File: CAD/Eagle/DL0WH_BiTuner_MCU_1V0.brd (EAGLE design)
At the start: 96.5 x 96.5 mm, 526 parts, among them Q0321 ABS07-32.768KHZ, Q1321 ABS07-32.768KHZ, Q2211 ABM3B-32.0000MHZ, Q2311 ABM3B-16.0000MHZ, T1051 MMBT2222, T1111 MMBT2222, T1121 MMBT2222, T1131 MMBT2222, U0111 STM32L4Z_144PIN_SMPS, U0521 PCAL6416APW, U0621 PCAL6416APW, U0711 IS25LP032D, U0721 IS25LP032D, U0801 CAT24C64, U0911 ZIO_EINK_1IN54, U1001 MIDAS_MCCOG21605B6W-FPTLWI, U1301 BNO085, U1401 BME680, U1501 LM4120IM5-3.0, U1511 MAX5217, U1531 CFPT-141-20MHZ, U1541 OPA354, U1542 LPV811, U1601 Si5338, U1651 TS5A23166, U1701 PCM1863, U1801 WM8523, U1901 SIM868, U2001 74LVC4245A, U2101 74LVC4245A, U2201 SX1262, U2271 PE4259, U2301 AX5243, U2401 LM53603-Q1, U2501 BQ24193, U2541 LPV811, U2601 BQ25570, U2681 TS5A23166, U2701 TPS62051, U2751 MCP4661-104E-MS, U2801 TS5A23166, U2901 TS5A23166, U3001 TS5A23166, U3101 TS5A23166, U3391 TS5A23166, U3392 TDK B4310, X1201 TTE_EN11-HSM, X1951 MICROSIM-8P_SDCARD-8P_MOLEX-1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, X2411 WIRE-TO-BOARD_5MM08_1X02, X2551 JST_S3B-XH-A, X2601 WIRE-TO-BOARD_5MM08_1X02, X3201 MOLEX 105017-0001, X3301 SMA_SMT_AMPHENOL-901-143, X3311 SAMTEC SMA-J-P-H-RA-TH1, X3371 SMA_SMT_AMPHENOL-901-143, SAM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, X3381 SMA_SMT_AMPHENOL-901-143, SAM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, X3391 SMA_SMT_AMPHENOL-901-143, SAM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, X3401 CUI SJ1-3535NS, X3411 CUI SJ1-3535NS, X3511 2X20/90_1MM27_HARWIN_M50-3202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, X3512 2X20/90_1MM27_HARWIN_M50-3202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, X3531 2X20/90_1MM27_HARWIN_M50-3202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, X3532 2X20/90_1MM27_HARWIN_M50-3202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

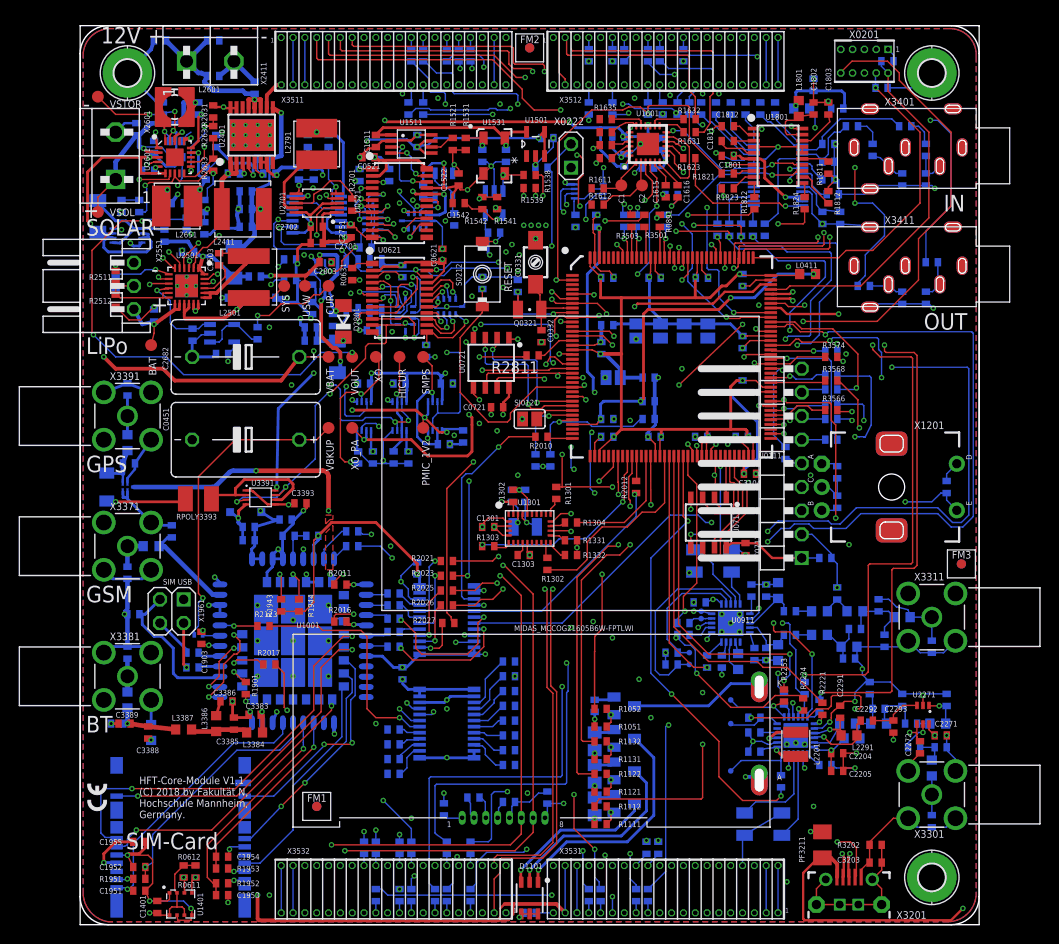
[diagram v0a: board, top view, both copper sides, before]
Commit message: HW_1V0 - CAD/Eagle - Initial setup of new PCB
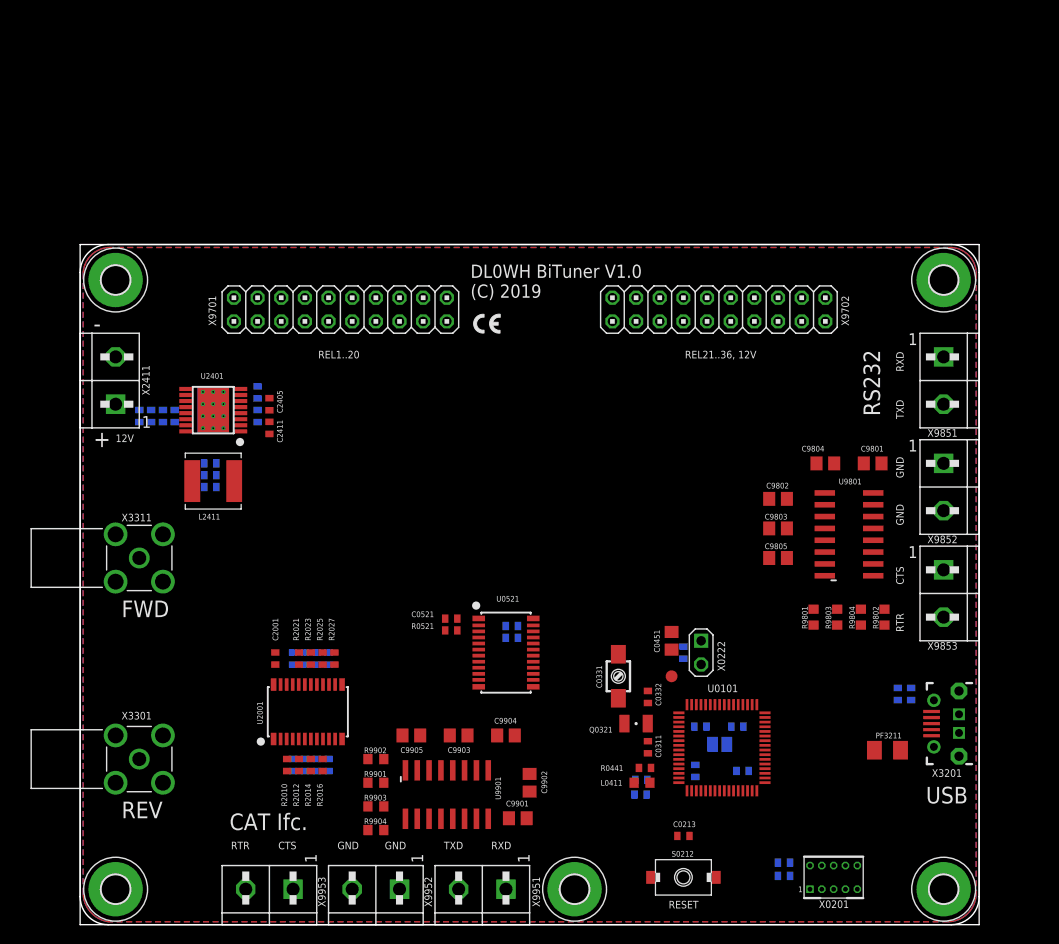
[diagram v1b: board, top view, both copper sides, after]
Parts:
- removed C0404, C0405, C0406, C0407, C0408, C0409, C0421, C0422, C0441, C0621, C0901, C1001, C1101, C1301, C1302, C1303, C1401, C1501, C1511, C1512, C1531, C1541, C1543, C1602, C1603, C1605, C1702, C1703, C1705, C1902, C2101, C2202, C2271, C2301, C2302, C2303, C2541, C2602, C2702, C2751, C2801, C2802, C2803, C2901, C2902, C2903, C3001, C3002, C3003, C3101, C3102, C3103, C3104, C3105, C3393: 100nF, df4iah_rcl:C0402
- removed C0423, C1801, C1802, C2606: 4.7uF, df4iah_rcl:C0402
- removed C0442, C1011, C1012, C1522, C1811, C1812, C1961, C2502, C2521: 1uF, df4iah_rcl:C0402
- removed C0711, C0721, C0801, C1601, C1604, C1951, C1955: 220nF, df4iah_rcl:C0402
- removed C1201, C1202, C1203, C1542, C2272: 1nF, df4iah_rcl:C0402
- removed C1321, C1322, C1952, C1953, C1954: 22pF, df4iah_rcl:C0402
- removed C1532: 100pF, df4iah_rcl:C0402
- removed C1615, C1616, C1712, C1722, C1903, C2603, C2605, C2653: 10nF, df4iah_rcl:C0402
- removed C1701, C1704, C1711, C1721, C1904, C2201, C2501, C2504, C2505, C2511, C2601, C2652, C2701: 10uF, df4iah_rcl:C0402
- removed C1706, C1803: 2.2uF, df4iah_rcl:C0402
- removed C1831, C1841: 2.7nF, df4iah_rcl:C0402
- removed C1901, C2204: 47pF, df4iah_rcl:C0402
- removed C2203: 470nF, df4iah_rcl:C0402
- removed C2205, C2503: 47nF, df4iah_rcl:C0402
- removed C2263, C2282, C2283: 3.3pF, df4iah_rcl:C0402
- removed C2264, C2281: 39pF, df4iah_rcl:C0402
- removed C2265, C2293, C3371, C3372, C3381, C3382, C3391, C3392: 0pF, df4iah_rcl:C0402
- removed C2266: 5.6pF, df4iah_rcl:C0402
- removed C2267: 2.2pF, df4iah_rcl:C0402
- removed C2291, C3386: 1.8pF, df4iah_rcl:C0402
- removed C2292: 2.4pF, df4iah_rcl:C0402
- removed C2312, C2313, C2316: N/A, df4iah_rcl:C0402
- removed C2314, C2315: 4.3pF, df4iah_rcl:C0402
- removed C2317, C2318, C2321, C2322, C2323: 4.7pF, df4iah_rcl:C0402
- removed C2682: 1F_6V_SCMR18H105MRBB0, df4iah_rcl:C115-080X160_POL
- removed C2703: 22uF, df4iah_rcl:C0402
- removed C2791: 6.8pF, df4iah_rcl:C0402
- removed C3383: 0.5pF, df4iah_rcl:C0402
- removed C3385, C3389: 1.2pF, df4iah_rcl:C0402
- removed C3388: 1.5pF, df4iah_rcl:C0402
- removed D1101: ASMT-YTB7-0AA02_RGB, df4iah_led:ASMT-YTB7_0AA02_RGB
- removed D1901: CMAD6001, df4iah_diode:SOD923
- removed D1902: MMSZ4690-E3-08 (5.6V), df4iah_diode:SOD123
- removed D2521, D2681, D2801, D2802: CRS08, df4iah_diode:SOD80C
- removed FM1, FM2, FM3: (no value), df4iah_fiducial:FIDUCIAL_MARK_1MM
- removed L1701, L1801: 10uH, df4iah_rcl:L0603
- removed L2201: 15uH, df4iah_rcl:L_3.00MM_X_3.00MM
- removed L2261: 0R, df4iah_rcl:L0603
- removed L2262: 47nH, df4iah_rcl:L0603
- removed L2263: 2.5nH, df4iah_rcl:L0603
- removed L2264, L3386, L3388: 4.7nH, df4iah_rcl:L0603
- removed L2282: 9.1nH, df4iah_rcl:L0603
- removed L2291: 15nH, df4iah_rcl:L0603
- removed L2311, L2316, L2317, L2321: 22nH, df4iah_rcl:L0603
- removed L2312, L2313: 100nH, df4iah_rcl:L0603
- removed L2314, L2315: 43nH, df4iah_rcl:L0603
- removed L2501: 2.2uH, df4iah_rcl:L_6.00MM_X_6.00MM
- removed L2601: 22uH, df4iah_rcl:WE-TPC_3MM8-3MM8_R-1MM3
- removed L2651, L2791: 10uH, df4iah_rcl:L_4.90MM_X_4.90MM
- removed L3384: 1.2nH, df4iah_rcl:L0603
- removed L3387: 2.7nH, df4iah_rcl:L0603
- removed L3393: WE-CBF_300R, rcl:L3216C
- removed Q1321: ABS07-32.768KHZ, df4iah_crystal:ABS07
- removed Q2211: ABM3B-32.0000MHZ, df4iah_crystal:ABM3B
- removed Q2311: ABM3B-16.0000MHZ, df4iah_crystal:ABM3B
- removed R0531, R0631, R0901, R0902, R0903, R0904, R1301, R1302, R1303, R1304, R1538, R1539, R1541, R1623, R1631, R1632, R1643, R1644, R1651, R1751, R1752, R1753, R1761, R1821, R1822, R1823, R1824, R1951, R1952, R1953, R2110, R2111, R2112, R2113, R2120, R2121, R2122, R2123, R2211, R2221, R2222, R2223, R2224, R2251, R2252, R2253, R2321, R2341, R2351, R2391, R2554, R2811, R3501, R3502, R3503, R3504, R3505, R3506, R3507, R3508, R3509, R3510, R3511, R3514, R3515, R3516, R3517, R3518, R3519, R3520, R3521, R3522, R3523, R3566, R3567, R3568, R3569, R3570, R3571, R3572, R3573, R3574, R3575, R3576, R3579, R3580, R3581, R3582, R3583, R3584, R3585, R3586, R3587, R3588: 47R, df4iah_rcl:R0402
- removed R0581, R0591, R0681, R0691: 1MR, df4iah_rcl:EXBD
- removed R0621, R1521, R2331, R2332, R2612, R2701, R2711: 100kR, df4iah_rcl:R0402
- removed R0891, R0892, R1811, R1812, R2521, R2651, R2681, R3512, R3513, R3577, R3578: 0R, df4iah_rcl:R0402
- removed R1031: 220kR, df4iah_rcl:R0402
- removed R1051, R1111, R1121, R1131: 1.5kR, df4iah_rcl:R0402
- removed R1052, R1112, R1122, R1132: 2.0kR, df4iah_rcl:R0402
- removed R1053: 27R, df4iah_rcl:R0402
- removed R1113, R1123, R1133: 27R, rcl:R0805
- removed R1331, R1332: 2kR, df4iah_rcl:R0402
- removed R1531, R1711, R1721, R1901, R1942: 10kR, df4iah_rcl:R0402
- removed R1542, R2803, R2804: 1MR, df4iah_rcl:R0402
- removed R1543, R2541: 33kR, df4iah_rcl:R0402
- removed R1611, R1612, R1635, R1636, R1661, R2114, R2115, R2116, R2117, R2124, R2125, R2126, R2127: N/A, df4iah_rcl:R0402
- removed R1712, R1722, R2801, R2802: 100R, df4iah_rcl:R0402
- removed R1731, R1741, R1742, R1743, R1744, R1745, R1746: D.C., df4iah_rcl:R0402
- removed R1831, R1841: 560R, df4iah_rcl:R0402
- removed R1941: NTC 10kR, df4iah_rcl:R0402
- removed R1943, R1944: 4.7kR, df4iah_rcl:R0402
- removed R1961, R1962: 22R, df4iah_rcl:R0402
- removed R2501: 240R, df4iah_rcl:R0402
- removed R2511: 2.27kR, df4iah_rcl:R0402
- removed R2512: 6.86kR, df4iah_rcl:R0402
- removed R2611: 1kR, df4iah_rcl:R0402
- removed R2621, R2633: 1.82MR, df4iah_rcl:R0402
- removed R2622: 10.0MR, df4iah_rcl:R0402
- removed R2631: 3.65MR, df4iah_rcl:R0402
- removed R2632: 7.50MR, df4iah_rcl:R0402
- removed R2641: 4.75MR, df4iah_rcl:R0402
- removed R2642: 8.20MR, df4iah_rcl:R0402
- removed R2712: 150kR, df4iah_rcl:R0402
- removed R3371, R3381, R3391: 0R, df4iah_rcl:R0603
- removed RPOLY3393: 50mA/150mA, rcl:R1210
- removed SJ0121, SJ0421, SJ0422, SJ0423, SJ0424: (no value), df4iah_jumper:SJ
- removed T1051, T1111, T1121, T1131: MMBT2222, transistor:SOT23
- removed TP_+1V1, TP_+1V2_MCU, TP_+3V3_HICUR, TP_+3V3_XO, TP_+3V3_XO_PA, TP_BQ_VBAT, TP_BQ_VOUT, TP_BQ_VSTOR, TP_IN_CLK1, TP_IN_CLK2, TP_LIPO_BAT, TP_LIPO_CUR, TP_LIPO_SYS, TP_VSOL, TP_VUSB_SW: PTR1B1,27, testpad:B1,27
- removed TP_AX_ADC1, TP_AX_ADC2, TP_AX_IRQ, TP_AX_TCXO_EN, TP_SX_DIO1, TP_SX_DIO2, TP_SX_DIO3: PTR1TP06R, testpad:TP06R
- removed U0111: STM32L4Z_144PIN_SMPS, df4iah_stm32l4:LQFP144
- removed U0621: PCAL6416APW, df4iah_dataconvertion:TSSOP24_SOT355-1
- removed U0711, U0721: IS25LP032D, df4iah_memory:SOIC8_150MIL
- removed U0801: CAT24C64, df4iah_memory:SOIC8_150MIL
- removed U0911: ZIO_EINK_1IN54, df4iah_lcd:ZIO_EINK_1IN54
- removed U1001: MIDAS_MCCOG21605B6W-FPTLWI, df4iah_lcd:MIDAS_MCCOG21605B6W-FPTLWI
- removed U1301: BNO085, df4iah_sensors:BNO085_LGA28
- removed U1401: BME680, df4iah_sensors:BME680
- removed U1501: LM4120IM5-3.0, df4iah_powersupply:SOT95P285X120-5N
- removed U1511: MAX5217, df4iah_dac:µMAX8
- removed U1531: CFPT-141-20MHZ, df4iah_osc:CFPT-141
- removed U1541: OPA354, df4iah_opamp:SOT-23-5
- removed U1542, U2541: LPV811, df4iah_opamp:SOT-23-5
- removed U1601: Si5338, df4iah_osc:QFN24_P0MM5_CTRPAD
- removed U1651, U2681, U2801, U2901, U3001, U3101, U3391: TS5A23166, df4iah_sc-switches:R-PDSO-G8
- removed U1701: PCM1863, df4iah_adc:R-PDSO-G30
- removed U1801: WM8523, df4iah_dac:TSSOP20
- removed U1901: SIM868, df4iah_gsm:SIM868
- removed U2101: 74LVC4245A, df4iah_dataconvertion:TSSOP24_SOT355-1
- removed U2201: SX1262, df4iah_rf:QFN24-4X4-0P5-PAD
- removed U2271: PE4259, df4iah_rf:SC-70_6-LEAD_2X1MM25_0P65
- removed U2301: AX5243, df4iah_rf:QFN20-4X4-0P5-PAD
- removed U2501: BQ24193, df4iah_powersupply:VQFN-24
- removed U2601: BQ25570, df4iah_powersupply:V-PVQFN-20
- removed U2701: TPS62051, df4iah_powersupply:S-PDSO-G10
- removed U2751: MCP4661-104E-MS, df4iah_dig-pot:TSSOP14
- removed U3392: TDK B4310, df4iah_rf:QCS5P
- removed X1201: TTE_EN11-HSM, df4iah_switch:TTE_EN11-HSM
- removed X1951: MICROSIM-8P_SDCARD-8P_MOLEX-104642-1610, df4iah_connector:MICROSIM-8P_SDCARD-8P_MOLEX-104642-1610
- removed X1961: (no value), df4iah_connector:2X02
- removed X2551: JST_S3B-XH-A, df4iah_connector:JST_S3B-XH-A
- removed X2601: WIRE-TO-BOARD_5MM08_1X02, df4iah_connector:WIRE-TO-BOARD_5MM08_1X02
- removed X3371, X3381, X3391: SMA_SMT_AMPHENOL-901-143, SAMTEC SMA-J-P-H-RA-TH1, df4iah_connector:SMA_SMT_AMPHENOL_901-143
- removed X3401, X3411: CUI SJ1-3535NS, df4iah_connector:SJ1-353XNS_3MM5-STEREO-AUDIO-JACKS
- removed X3511, X3512, X3531, X3532: 2X20/90_1MM27_HARWIN_M50-3202045_SOCKET, df4iah_connector:2X20/90_1MM27_HARWIN_M50-3202045_SOCKET
- added C9801, C9802, C9803, C9804, C9805, C9901, C9902, C9903, C9904, C9905: 1uF, rcl:C0805
- added H3651, H3661: MOUNT-PAD-ROUND3.0, df4iah_holes:3,0-PAD
- added R9801, R9802, R9803, R9804, R9901, R9902, R9903, R9904: 47R, df4iah_rcl:R0603
- added U0101: STM32L476RXT_64PIN_LDO, df4iah_stm32l4:LQFP64
- added U9801, U9901: MAX232_SOIC16, df4iah_dataconvertion:SOIC16N
- added X9701, X9702: (no value), df4iah_connector:2X10
- added X9851, X9852, X9853, X9951, X9952, X9953: WIRE-TO-BOARD_5MM08_1X02, df4iah_connector:WIRE-TO-BOARD_5MM08_1X02
- C0451: value 1F_6V_SCMR18H105MRBB0 -> 47uF; device df4iah_rcl:C115-080X160_POL -> df4iah_rcl:C0805
- H3611, H3621, H3631: value MOUNT-PAD-ROUND2.8 -> MOUNT-PAD-ROUND3.0; device holes:2,8-PAD -> df4iah_holes:3,0-PAD
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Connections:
- removed net +1V2: C2703.1, C2791.2, C3101.1, L2791.1, TP_+1V1.TP, U2751.8, U3101.1, U3101.5
- removed net +1V5_UNUSED: SJ0424.2
- removed net +1V8_UNUSED: SJ0423.2
- removed net +2V5_UNUSED: SJ0422.2
- removed net +3V0_20MHZ_VCTCXO: C1511.1, C1531.1, U1501.5, U1511.1, U1531.4
- removed net +3V3_GPS: RPOLY3393.1, U3391.2, U3391.6
- removed net +3V3_HICUR: C1601.1, C1602.1, C1603.1, C1604.1, C1605.2, C1701.1, C1702.1, C1801.1, C3003.1, L1701.2, L1801.2, TP_+3V3_HICUR.TP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
- removed net +3V3_XO: C1501.1, C1512.1, C2903.1, TP_+3V3_XO.TP, U1501.3, U1501.4, U1511.5, U1511.7, U2901.6
- removed net +3V3_XO_PA: C1541.1, TP_+3V3_XO_PA.TP, U1541.5, U2901.2
- removed net +5V0: C2521.2, D2521.C, R2521.2, R2681.2, U2501.1, U2501.24, X3511.37, X3511.38, X3531.37, X3531.38
- removed net 20MHZ_DAC_OUT: R1521.1, U1511.6
- removed net 20MHZ_XO: R1538.1, U1531.3, U1541.3
- removed net 20MHZ_XON: C1616.1, R1539.2, R1661.1
- removed net 20MHZ_XOP: C1615.1, R1538.2, R1661.2
- removed net AD_VCTCXO1: R1543.1, U1542.1, U1542.4
- removed net AUDIOADC_AVDD: C1703.2, L1701.1, U1701.8
- removed net AUDIOADC_BCK: R1752.1, U1701.17
- removed net AUDIOADC_DOUT: R1751.1, U1701.18
- removed net AUDIOADC_INTA: R1761.1, U1701.21
- removed net AUDIOADC_LDO: C1704.1, C1705.1, U1701.11
- removed net AUDIOADC_LRCK: R1753.1, U1701.16
- removed net AUDIOADC_MIC_BIAS: R1731.2, U1701.5
- removed net AUDIOADC_VINL1: C1712.1, R1712.2, U1701.3
- removed net AUDIOADC_VINL1_R: C1711.2, R1712.1
- removed net AUDIOADC_VINL2: R1741.2, U1701.1
- removed net AUDIOADC_VINL3: R1743.2, U1701.29
- removed net AUDIOADC_VINL4: R1745.2, U1701.27
- removed net AUDIOADC_VINR1: C1722.1, R1722.2, U1701.4
- removed net AUDIOADC_VINR1_R: C1721.2, R1722.1
- removed net AUDIOADC_VINR2: R1742.2, U1701.2
- removed net AUDIOADC_VINR3: R1744.2, U1701.30
- removed net AUDIOADC_VINR4: R1746.2, U1701.28
- removed net AUDIOADC_VREF: C1706.1, U1701.6
- removed net AUDIO_DAC_A0: R1811.2, U1801.15
- removed net AUDIO_DAC_A1: R1812.2, U1801.12
- removed net AUDIO_DAC_AVDD: C1802.2, L1801.1, U1801.19
- removed net AUDIO_DAC_BCLK: R1822.2, U1801.10
- removed net AUDIO_DAC_CPCA: C1811.1, U1801.5
- removed net AUDIO_DAC_CPCB: C1811.2, U1801.3
- removed net AUDIO_DAC_CPVOUTN: C1812.2, U1801.2
- removed net AUDIO_DAC_DACDAT: R1821.2, U1801.8
- removed net AUDIO_DAC_LINEVOUTL: R1831.1, U1801.1
- removed net AUDIO_DAC_LINEVOUTR: R1841.1, U1801.20
- removed net AUDIO_DAC_LRCLK: R1823.2, U1801.9
- removed net AUDIO_DAC_MCLK: R1824.2, U1801.11
- removed net AUDIO_DAC_VMID: C1803.2, U1801.18
- removed net AUDIO_IN_L: C1711.1, R1711.2, X3401.12, X3401.22
- removed net AUDIO_IN_R: C1721.1, R1721.2, X3401.13, X3401.23
- removed net AUDIO_OUT_L: C1831.1, R1831.2, X3411.12, X3411.22
- removed net AUDIO_OUT_R: C1841.1, R1841.2, X3411.13, X3411.23
- removed net AX_8MHZ: R2321.2, U1601.4
- removed net AX_ADC1: R2331.1, TP_AX_ADC1.TP, U2301.17
- removed net AX_ADC2: R2332.1, TP_AX_ADC2.TP, U2301.18
- removed net AX_ANTN: C2313.1, C2315.1, L2313.1, U2301.4
- removed net AX_ANTP: C2312.1, C2314.1, L2312.1, U2301.3
- removed net AX_B1: C2317.1, L2314.2, L2317.1
- removed net AX_B2: C2316.1, C2318.1, L2315.2, L2316.2
- removed net AX_CLK16A: Q2311.1, U2301.20
- removed net AX_CLK16B: Q2311.3, U2301.19
- removed net AX_COMB: C2318.2, C2321.1, C2322.1, L2317.2, L2321.1
- removed net AX_IRQ: R2351.2, TP_AX_IRQ.TP, U2301.14
- removed net AX_L1: L2311.1, U2301.8
- removed net AX_L2: L2311.2, U2301.7
- removed net AX_SYSCLK: R2321.1, U2301.9
- removed net AX_T1: C2314.2, L2314.1
- removed net AX_T2: C2315.2, L2315.1
- removed net AX_VDD1: C2302.2, U2301.1
- removed net AX_VDD5: C2303.2, U2301.5
- removed net BNO085_CAP: C1303.1, U1301.9
- removed net BNO085_CLKSEL1_XOUT32: C1322.1, Q1321.1, U1301.26
- removed net BNO085_ENV_SCL: R1332.1, U1301.15
- removed net BNO085_ENV_SDA: R1331.1, U1301.16
- removed net BNO085_H_CSN: R1304.2, U1301.18
- removed net BNO085_INTN: R1302.2, U1301.14
- removed net BNO085_MISO: R1301.2, U1301.20
- removed net BNO085_PS0_WAKE: R1303.2, U1301.6
- removed net BNO085_XIN32: C1321.1, Q1321.2, U1301.27
- removed net BQ_LBOOST: L2601.1, R2612.2, U2601.20
- removed net BQ_LBUCK: L2651.2, U2601.16
- removed net BQ_OK_HYST: R2632.2, R2633.1, U2601.10
- removed net BQ_OK_PROG: R2631.2, R2632.1, U2601.11
- removed net BQ_VBAT: C2682.+, TP_BQ_VBAT.TP, U2601.18, U2681.8
- removed net BQ_VBAT_OV: R2621.2, R2622.1, U2601.7
- removed net BQ_VOUT: C2652.1, C2653.1, L2651.1, R2651.1, TP_BQ_VOUT.TP, U2601.14
- removed net BQ_VOUT_SET: R2641.2, R2642.1, U2601.12
- removed net BQ_VRDIFF: R2622.2, R2633.2, R2642.2, U2601.8
- removed net BQ_VREF_SAMP: C2603.2, U2601.4
- removed net BQ_VSTOR: C2605.1, C2606.1, D2681.C, TP_BQ_VSTOR.TP, U2601.19, U2601.3, U2601.6, U2681.2, U2681.3, U2681.6, U2681.7
- removed net BQ_VSTOR_SW: D2681.A, R2681.1, U2681.1, U2681.5
- removed net BT_ANT: C3382.1, R3381.2, X3381.1
- removed net CH1_ANT: C2283.2, L2282.1, X3301.1
- removed net CH2_ANT: C2321.2, C2323.1, L2321.2, X3311.1
- removed net CLK0_N: R1643.2, X3532.4
- removed net CLK0_P: R1644.2, X3532.3
- removed net CLK2_N: R1631.2, X3512.4
- removed net CLK2_P: R1632.2, X3512.3
- removed net CLK_AUDIO_ADC: R1623.1, U1701.15
- removed net EINK_BUSY_R: R0904.2, U0911.8
- removed net EINK_CS_R: R0901.2, U0911.5
- removed net EINK_D/C_R: R0902.2, U0911.6
- removed net EINK_RESET_R: R0903.2, U0911.7
- removed net EVT_N_OUT: R3509.2, X3511.29
- removed net EVT_S_OUT: R3574.2, X3531.29
- removed net GPS_ANT: C3392.1, R3391.2, X3391.1
- removed net GPS_ANT_SAW: C3391.1, L3393.1, R3391.1, U3392.4
- removed net GPS_POLY: L3393.2, RPOLY3393.2
- removed net GSM_ANT: C3372.1, R3371.2, X3371.1
- removed net I2C1_SCL: R0612.1, R0891.1, U0521.22, U0621.22, U0801.6, U1001.7, U1401.4, U1511.3, U1601.12, U1701.24, U1801.14, U2501.5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
- removed net I2C1_SDA: R0611.1, R0892.1, U0521.23, U0621.23, U0801.5, U1001.6, U1401.3, U1511.4, U1601.19, U1701.23, U1801.13, U2501.6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
- removed net I2C2_SCL_N: R3512.2, X3512.7
- removed net I2C2_SCL_S: R3577.2, X3532.7
- removed net I2C2_SDA_N: R3513.2, X3512.8
- removed net I2C2_SDA_S: R3578.2, X3532.8
- removed net I2S_FS_N_IN: R3523.2, X3512.26
- removed net I2S_FS_N_OUT: R3520.2, X3512.20
- removed net I2S_FS_S_IN: R3588.2, X3532.26
- removed net I2S_FS_S_OUT: R3585.2, X3532.20
- removed net I2S_MCLK_N_OUT: R3519.2, X3512.19
- removed net I2S_MCLK_S_OUT: R3584.2, X3532.19
- removed net I2S_SCK_N_IN: R3521.2, X3512.23
- removed net I2S_SCK_N_OUT: R3517.2, X3512.17
- removed net I2S_SCK_S_IN: R3586.2, X3532.23
- removed net I2S_SCK_S_OUT: R3582.2, X3532.17
- removed net I2S_SD_N_IN: R3522.2, X3512.24
- removed net I2S_SD_N_OUT: R3518.2, X3512.18
- removed net I2S_SD_S_IN: R3587.2, X3532.24
- removed net I2S_SD_S_OUT: R3583.2, X3532.18
- removed net LCD_BL_K: T1051.3, U1001.11
- removed net LCD_CAP1N: C1011.2, U1001.2
- removed net LCD_CAP1P: C1011.1, U1001.3
- removed net LCD_VOUT: C1012.1, U1001.1
- removed net LED_B_B: R1051.2, R1052.1, T1051.1
- removed net LED_B_B1: R1131.2, R1132.1, T1131.1
- removed net LED_B_E: R1053.2, T1051.2
- removed net LED_B_E1: R1133.2, T1131.2
- removed net LED_B_K1: D1101.1, T1131.3
- removed net LED_G_B1: R1121.2, R1122.1, T1121.1
- removed net LED_G_E1: R1123.2, T1121.2
- removed net LED_G_K1: D1101.2, T1121.3
- removed net LED_R_B1: R1111.2, R1112.1, T1111.1
- removed net LED_R_E1: R1113.2, T1111.2
- removed net LED_R_K1: D1101.3, T1111.3
- removed net LIPO_ADC_CUR_IN_LOOP: R2541.2, U2541.1, U2541.4
- removed net LIPO_BAT: C2511.1, TP_LIPO_BAT.TP, U2501.13, U2501.14, X2551.1
- removed net LIPO_BTST: C2503.1, U2501.21
- removed net LIPO_ILIM: R2501.2, U2501.10, U2541.3
- removed net LIPO_INT: R2554.2, U2501.7
- removed net LIPO_PMID: C2501.1, U2501.23
- removed net LIPO_REGN: C2502.1, R2511.2, U2501.22
- removed net LIPO_SW: C2503.2, L2501.2, U2501.19, U2501.20
- removed net LIPO_SYS: C1901.2, C1902.2, C1904.2, C2504.1, C2505.1, D1902.C, L2501.1, TP_LIPO_SYS.TP, U1901.34, U1901.35, U2501.15, U2501.16
- removed net LIPO_TS12: R2511.1, R2512.1, U2501.11, U2501.12, X2551.2
- removed net LS2_B12: R2124.1, U2101.17
- removed net LS2_B13: R2125.1, U2101.16
- removed net LS2_B14: R2126.1, U2101.15
- removed net LS2_B15: R2127.1, U2101.14
- removed net LS2_B4: R2114.2, U2101.7
- removed net LS2_B4_R: R2124.2
- removed net LS2_B5: R2115.2, U2101.8
- removed net LS2_B5_R: R2125.2
- removed net LS2_B6: R2116.2, U2101.9
- removed net LS2_B6_R: R2126.2
- removed net LS2_B7: R2117.2, U2101.10
- removed net LS2_B7_R: R2127.2
- removed net MCP4661_P0B_P1W: U2751.10, U2751.6
- removed net MCU_AX_MISO: R2341.2, U2301.12
- removed net MCU_AX_SEL_OUT: R2391.2, U2301.10
- removed net MCU_HSE_R: R1651.2, U1651.2, U1651.5
- removed net MCU_RF_SYNC_IN_R: R2113.2, U2101.6
- removed net MCU_SPI3_MOSI: R2223.2, U0911.3, U1301.17, U2201.17, U2301.13
- removed net MCU_SPI3_SCK: R2222.2, U0911.4, U1301.19, U2201.18, U2301.11
- removed net MCU_SX_SEL_OUT: R2221.2, U2201.19
- removed net MCU_VBUS_SOFT_SW_EN_OUT_R: R2803.1, R2811.2, U2801.7
- removed net MCU_VDD12: C3103.1, C3104.2, C3105.1, TP_+1V2_MCU.TP, U0111.142, U0111.70, U3101.2, U3101.6
- removed net MCU_VDDIO2: C0421.2, C0422.1, C0423.1, SJ0421.1, SJ0422.1, SJ0423.1, SJ0424.1, U0111.131, U0111.95
- removed net MCU_VREF_P: C0441.2, C0442.2, U0111.32
- removed net MCU_VSSA: SJ0121.2, U0111.30
- removed net MC_SW: X1951.SW
- removed net PD0: U0111.114
- removed net PD1: R3516.1, R3581.1, U0111.115
- removed net PD10: R3567.1, U0111.79
- removed net PD11: R1751.2, R3522.1, R3587.1, U0111.80
- removed net PD12: R1753.2, R3523.1, R3588.1, U0111.81
- removed net PD13: U0111.82
- removed net PD14: R3568.1, U0111.85
- removed net PD15: R3569.1, U0111.86
- removed net PD3: R3515.1, R3580.1, U0111.117
- removed net PD4: U0111.118
- removed net PD5: U0111.119
- removed net PD6: U0111.122
- removed net PD7: U0111.123, U0721.7
- removed net PD8: R2211.1, U0111.77
- removed net PD9: R3566.1, U0111.78
- removed net PE0: U0111.140
- removed net PE1: U0111.141
- removed net PE10: R1824.1, R3519.1, R3584.1, U0111.63
- removed net PE11: U0111.64, U0711.1, U0721.1
- removed net PE12: U0111.65, U0711.5
- removed net PE13: U0111.66, U0711.2
- removed net PE14: U0111.67, U0711.3
- removed net PE15: U0111.68, U0711.7
- removed net PE2: U0111.1
- removed net PE3: R1821.1, R3518.1, R3583.1, U0111.2
- removed net PE4: U0111.3
- removed net PE5: U0111.4
- removed net PE6: R1052.2, U0111.5
- removed net PE7: R2351.1, U0111.58
- removed net PE8: R1822.1, R3517.1, R3582.1, U0111.59
- removed net PE9: R1823.1, R3520.1, R3585.1, U0111.60
- removed net PEXPA_INTN: R0531.2, U0521.1
- removed net PEXPB_INTN: R0631.2, U0621.1
- removed net PEXPB_P0_0_R: R0681.2, U0621.4, U2701.4
- removed net PEXPB_P0_1_R: R0681.3, U0621.5, U2701.2
- removed net PEXPB_P0_2_R: R0681.4, U0621.6, U2501.4
- removed net PEXPB_P0_3_R: R0681.5, U0621.7, U2501.3
- removed net PEXPB_P0_4_R: R0681.7, U0621.8, U1801.7
- removed net PEXPB_P0_5_R: R0681.8, TP_AX_TCXO_EN.TP, U0621.9, U2301.15
- removed net PEXPB_P0_6_R: R0681.9, U0621.10
- removed net PEXPB_P0_7_R: R0681.10, U0621.11, U3391.3, U3391.7
- removed net PEXPB_P1_0: R2121.1, U2101.20
- removed net PEXPB_P1_0_R: R0691.2, R2121.2, U0621.13
- removed net PEXPB_P1_1: R2110.2, U2101.3
- removed net PEXPB_P1_1_R: R0691.3, R2110.1, U0621.14
- removed net PEXPB_P1_2: R2112.2, U2101.5
- removed net PEXPB_P1_2_R: R0691.4, R2112.1, U0621.15
- removed net PEXPB_P1_3_R: R0691.5, R0903.1, U0621.16
- removed net PEXPB_P1_4_R: R0691.7, U0621.17
- removed net PEXPB_P1_5_R: C1201.1, R0691.8, U0621.18, X1201.A
- removed net PEXPB_P1_6_R: C1202.1, R0691.9, U0621.19, X1201.B
- removed net PEXPB_P1_7_R: C1203.1, R0691.10, U0621.20, X1201.E
- removed net PEXPB_RESET: R0621.1, U0621.3
- removed net PE_RFC: C2281.1, U2271.5
- removed net PE_RFC_2: C2281.2, C2282.2, L2282.2
- removed net PF0: R3513.1, R3578.1, U0111.10
- removed net PF1: R3512.1, R3577.1, U0111.11
- removed net PF10: U0111.22, U0711.6, U0721.6
- removed net PF11: R1304.1, U0111.49
- removed net PF12: C2272.1, R2252.2, U0111.50, U2271.4
- removed net PF13: R1302.1, U0111.53
- removed net PF14: R2391.1, U0111.54
- removed net PF15: R2221.1, U0111.55
- removed net PF2: U0111.12
- removed net PF3: R0531.1, U0111.13
- removed net PF4: R0631.1, U0111.14
- removed net PF5: R2811.1, U0111.15
- removed net PF6: R3510.1, U0111.18
- removed net PF7: R2612.1, U0111.19
- removed net PF8: R3575.1, U0111.20
- removed net PF9: R2027.2, U0111.21
- removed net PG0: R2253.2, U0111.56
- removed net PG1: R2251.2, U0111.57
- removed net PG10: R3506.1, R3571.1, U0111.125
- removed net PG11: R3508.1, R3573.1, U0111.126
- removed net PG12: R3507.1, R3572.1, U0111.127
- removed net PG13: R0892.2, U0111.128
- removed net PG14: R0891.2, U0111.129
- removed net PG2: U0111.87
- removed net PG3: R0901.1, U0111.88
- removed net PG4: R3509.1, R3574.1, U0111.89
- removed net PG5: R0902.1, U0111.90
- removed net PG6: R2025.2, U0111.91
- removed net PG7: R2014.1, U0111.92
- removed net PG8: R2021.2, U0111.93
- removed net PG9: R3505.1, R3570.1, U0111.124
- removed net PN00: R3501.2, X3511.7
- removed net PN01: R3502.2, X3511.9
- removed net PN02: R3503.2, X3511.11
- removed net PN03: R3504.2, X3511.13
- removed net PS00: R3566.2, X3531.7
- removed net PS01: R3567.2, X3531.9
- removed net PS02: R3568.2, X3531.11
- removed net PS03: R3569.2, X3531.13
- removed net S6: X1951.S6
- removed net SC_2: R1951.2, X1951.S2
- removed net SC_3: R1952.2, X1951.S3
- removed net SC_7: R1953.1, X1951.S7
- removed net SI5338_CLK0A: R1644.1, U1601.22
- removed net SI5338_CLK0B: R1643.1, U1601.21
- removed net SI5338_CLK1A: R1636.1, U1601.18
- removed net SI5338_CLK1B: R1635.1, U1601.17
- removed net SI5338_CLK2A: R1632.1, U1601.14
- removed net SI5338_CLK2B: R1631.1, U1601.13
- removed net SI5338_CLK3A: U1601.10, U1651.1
- removed net SI5338_CLK3B: R1623.2, U1601.9
- removed net SI5338_IN5: C1615.2, U1601.5
- removed net SI5338_IN6: C1616.2, U1601.6
- removed net SI5338_IN_CLK1: R1611.1
- removed net SI5338_IN_CLK1_R: R1611.2, TP_IN_CLK1.TP, U1601.1
- removed net SI5338_IN_CLK2: R1612.1
- removed net SI5338_IN_CLK2_R: R1612.2, TP_IN_CLK2.TP, U1601.2
- removed net SI5338_OUT_CLK1_N: R1635.2
- removed net SI5338_OUT_CLK1_P: R1636.2
- removed net SIM_!PWRKEY: R2111.1, U1901.39
- removed net SIM_1PPS: R2017.1, U1901.60
- removed net SIM_ADC: R1941.2, R1942.1, U1901.38
- removed net SIM_BT_ANT: C3383.1, L3384.1, U1901.20
- removed net SIM_BT_ANT_L: C3385.1, L3384.2, L3386.1, L3387.1
- removed net SIM_BT_ANT_L_L: C3381.1, C3388.1, C3389.1, L3387.2, R3381.1
- removed net SIM_BT_ANT_L_LC: C3386.1, L3386.2
- removed net SIM_BT_ANT_L_L_LC: C3388.2, L3388.1
- removed net SIM_GNSS_EN: R1901.2, U1901.59
- removed net SIM_GPIO1: R1901.1, U1901.57
- removed net SIM_GPIO2: U1901.58
- removed net SIM_GPS_ANT: U1901.68, U3392.1
- removed net SIM_GPS_RXD: U1901.22, U1901.62
- removed net SIM_GPS_TXD: U1901.23, U1901.61
- removed net SIM_GSM_ANT: C3371.1, R3371.1, U1901.32
- removed net SIM_MCCA0: U1901.49, X1951.T7
- removed net SIM_MCCA1: U1901.48, X1951.T8
- removed net SIM_MCCA2: U1901.47, X1951.T1
- removed net SIM_MCCA3: U1901.46, X1951.T2
- removed net SIM_MCCCK: U1901.50, X1951.T5
- removed net SIM_MCCM0: U1901.51, X1951.T3
- removed net SIM_MICN: U1901.10
- removed net SIM_MICP: U1901.9
- removed net SIM_NETLIGHT: R2122.2, U1901.41
- removed net SIM_NETLIGHT_R: R2122.1, U2101.19
- removed net SIM_PWRKEY_R: R2111.2, U2101.4
- removed net SIM_RF_SYNC: R2123.2, U1901.29
- removed net SIM_RF_SYNC_R: R2123.1, U2101.18
- removed net SIM_SCL: R1944.1, U1901.65
- removed net SIM_SDA: R1943.1, U1901.64
- removed net SIM_SIM1_CLK: C1953.2, R1952.1, U1901.16
- removed net SIM_SIM1_DATA: C1954.2, R1953.2, U1901.15
- removed net SIM_SIM1_DET: U1901.14
- removed net SIM_SIM1_RST: C1952.2, R1951.1, U1901.17
- removed net SIM_SIM1_VDD: C1951.1, U1901.18, X1951.S1
- removed net SIM_SIM2_CLK: U1901.54
- removed net SIM_SIM2_DATA: U1901.53
- removed net SIM_SIM2_DET: U1901.52
- removed net SIM_SIM2_RST: U1901.55
- removed net SIM_SIM2_VDD: U1901.56
- removed net SIM_SPK1N: U1901.12
- removed net SIM_SPK1P: U1901.11
- removed net SIM_SPK2N: U1901.43
- removed net SIM_SPK2P: U1901.44
- removed net SIM_STATUS: R2120.2, U1901.42
- removed net SIM_STATUS_R: R2120.1, U2101.21
- removed net SIM_UART1_CTS: R2013.1, U1901.4
- removed net SIM_UART1_DCD: R2016.1, U1901.5
- removed net SIM_UART1_DTR: R2024.2, U1901.6
- removed net SIM_UART1_RI: R2015.1, U1901.7
- removed net SIM_UART1_RTS: R2022.2, U1901.3
- removed net SIM_UART1_RXD: R2020.2, U1901.2
- removed net SIM_UART1_TXD: R2011.1, U1901.1
- removed net SIM_USBCON_DM: R1961.2, X1961.4
- removed net SIM_USBCON_DP: R1962.2, X1961.2
- removed net SIM_USB_DM: R1961.1, U1901.26
- removed net SIM_USB_DP: R1962.1, U1901.25
- removed net SIM_USB_VBUS: C1961.2, U1901.24, X1961.3
- removed net SIM_VRTC: C1903.2, D1901.C, U1901.28
- removed net SPI2_MISO_N: R3515.2, X3512.12
- removed net SPI2_MISO_S: R3580.2, X3532.12
- removed net SPI2_MOSI_N: R3514.2, X3512.11
- removed net SPI2_MOSI_S: R3579.2, X3532.11
- removed net SPI2_SCK_N: R3516.2, X3512.13
- removed net SPI2_SCK_S: R3581.2, X3532.13
- removed net SX_BUSY: R2211.2, U2201.14
- removed net SX_DCC_SW: L2201.1, U2201.9
- removed net SX_DIO1: R2253.1, TP_SX_DIO1.TP, U2201.13
- removed net SX_DIO2: R2252.1, TP_SX_DIO2.TP, U2201.12
- removed net SX_DIO3: R2251.1, TP_SX_DIO3.TP, U2201.6
- removed net SX_MISO: R2224.2, U2201.16
- removed net SX_RFI_2: C2292.2, C2293.2, U2271.3
- removed net SX_RFI_N: C2292.1, L2291.1, U2201.22
- removed net SX_RFI_P: C2291.2, L2291.2, U2201.21
- removed net SX_RFO: L2261.2, U2201.23
- removed net SX_RFO_2: C2263.1, C2265.2, L2261.1, L2262.1, L2263.2
- removed net SX_RFO_3: C2263.2, C2264.1, C2266.1, L2263.1
- removed net SX_RFO_4: C2264.2, L2264.2
- removed net SX_RFO_5: C2267.1, L2264.1, U2271.1
- removed net SX_VREG: C2203.1, L2201.2, U2201.7
- removed net SX_VR_PA: C2204.1, C2205.1, L2262.2, U2201.24
- removed net SX_XTA: Q2211.1, U2201.3
- removed net SX_XTB: Q2211.3, U2201.4
- removed net TIMCAP_N_IN: R3510.2, X3511.31
- removed net TIMCAP_S_IN: R3575.2, X3531.31
- removed net U3311_B4_R: R2114.1
- removed net U3311_B5_R: R2115.1
- removed net U3311_B6_R: R2116.1
- removed net U3311_B7_R: R2117.1
- removed net UART1_CTS_N_IN: R3508.2, X3511.26
- removed net UART1_CTS_S_IN: R3573.2, X3531.26
- removed net UART1_RTS_N_OUT: R3507.2, X3511.25
- removed net UART1_RTS_S_OUT: R3572.2, X3531.25
- removed net UART1_RX_N_IN: R3506.2, X3511.24
- removed net UART1_RX_S_IN: R3571.2, X3531.24
- removed net UART1_TX_N_OUT: R3505.2, X3511.23
- removed net UART1_TX_S_OUT: R3570.2, X3531.23
- removed net VCTCXO_PA_N: C1542.1, R1542.1, U1541.4
- removed net VCTCXO_PA_O: R1541.1, R1542.2, U1541.1
- removed net VDD12_EN: R2701.2, U2701.8
- removed net VDD12_FB: C2791.1, U2701.5, U2751.9
- removed net VDD12_LBI: R2711.2, R2712.1, U2701.6
- removed net VDD12_SW: L2791.2, U2701.9
- removed net VDDUSB_DK: C2802.1, D2801.C, D2802.C, R2801.2, R2802.2, R2803.2, U2801.8
- removed net VDDUSB_SOFT: R2801.1, R2802.1, U2801.1
- removed net VSOL: C2601.1, C2602.1, L2601.2, R2611.1, TP_VSOL.TP, U2601.2, X2601.1
- removed net VUSB_SW: C2803.1, D2802.A, R2521.1, TP_VUSB_SW.TP, U2801.2, U2801.6
- removed net WAKEUP_N_IN: R3511.2, X3511.33
- removed net WAKEUP_S_IN: R3576.2, X3531.33
- removed net XO_LP: C1522.1, R1521.2, R1531.1, U1542.3
- removed net XO_OUT: R1541.2, U1651.6
- removed net XO_VC: C1532.1, R1531.2, U1531.1
- new net +12V: X9702.17, X9702.18, X9702.19, X9702.20
- new net +5V: C9801.1, C9901.1, U9801.16, U9901.16
- new net CAT_DTE_CTS: U9901.7, X9953.1
- new net CAT_DTE_RTR: U9901.8, X9953.2
- new net CAT_DTE_RXD: U9901.14, X9951.1
- new net CAT_DTE_TXD: U9901.13, X9951.2
- new net CAT_MX_C1N: C9902.2, U9901.3
- new net CAT_MX_C1P: C9902.1, U9901.1
- new net CAT_MX_C2M: C9903.2, U9901.5
- new net CAT_MX_C2P: C9903.1, U9901.4
- new net CAT_MX_VM: C9905.1, U9901.6
- new net CAT_MX_VP: C9904.1, U9901.2
- new net MCU_I2C1_SCL: R0612.1, U0521.22
- new net MCU_I2C1_SDA: R0611.1, U0521.23
- new net MP_CAT_CTS_R: R9903.2, U9901.10
- new net MP_CAT_RTR_R: R9904.2, U9901.9
- new net MP_CAT_RXD_R: R9901.2, U9901.11
- new net MP_CAT_TXD_R: R9902.2, U9901.12
- new net MP_RS_CTS_R: R9803.2, U9801.10
- new net MP_RS_RTR_R: R9804.2, U9801.9
- new net MP_RS_RXD_R: R9801.2, U9801.11
- new net MP_RS_TXD_R: R9802.2, U9801.12
- new net N$1: R9901.1
- new net N$2: C2001.1, U2001.23, U2001.24
- new net N$3: R9902.1
- new net N$4: R9903.1
- new net N$5: R9904.1
- new net N$6: R9801.1
- new net N$7: R9802.1
- new net N$8: R9803.1
- new net N$9: R9804.1
- new net PA11: U0101.44
- new net PA12: U0101.45
- new net PB11: U0101.30
- new net RELAIS1: X9701.1
- new net RELAIS10: X9701.10
- new net RELAIS11: X9701.11
- new net RELAIS12: X9701.12
- new net RELAIS13: X9701.13
- new net RELAIS14: X9701.14
- new net RELAIS15: X9701.15
- new net RELAIS16: X9701.16
- new net RELAIS17: X9701.17
- new net RELAIS18: X9701.18
- new net RELAIS19: X9701.19
- new net RELAIS2: X9701.2
- new net RELAIS20: X9701.20
- new net RELAIS21: X9702.1
- new net RELAIS22: X9702.2
- new net RELAIS23: X9702.3
- new net RELAIS24: X9702.4
- new net RELAIS25: X9702.5
- new net RELAIS26: X9702.6
- new net RELAIS27: X9702.7
- new net RELAIS28: X9702.8
- new net RELAIS29: X9702.9
- new net RELAIS3: X9701.3
- new net RELAIS30: X9702.10
- new net RELAIS31: X9702.11
- new net RELAIS32: X9702.12
- new net RELAIS33: X9702.13
- new net RELAIS34: X9702.14
- new net RELAIS35: X9702.15
- new net RELAIS36: X9702.16
- new net RELAIS4: X9701.4
- new net RELAIS5: X9701.5
- new net RELAIS6: X9701.6
- new net RELAIS7: X9701.7
- new net RELAIS8: X9701.8
- new net RELAIS9: X9701.9
- new net RM_BCK: X3311.1
- new net RM_FWD: X3301.1
- new net RS_DTE_CTS: U9801.7, X9853.1
- new net RS_DTE_RTR: U9801.8, X9853.2
- new net RS_DTE_RXD: U9801.14, X9851.1
- new net RS_DTE_TXD: U9801.13, X9851.2
- new net RS_MX_C1N1: C9802.2, U9801.3
- new net RS_MX_C1P: C9802.1, U9801.1
- new net RS_MX_C2M1: C9803.2, U9801.5
- new net RS_MX_C2P: C9803.1, U9801.4
- new net RS_MX_VM: C9805.1, U9801.6
- new net RS_MX_VP: C9804.1, U9801.2
- net +3V3: no longer C0621.1, C0711.1, C0721.1, C0801.1, C0901.1, C1001.1, C1101.1, C1301.1, C1302.1, C1401.1, C1543.1, C2201.1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
- net GND: now also C0451.2, C9801.2, C9804.2, C9805.2, C9901.2, C9904.2, C9905.2, H3611.B3,0, H3621.B3,0, H3631.B3,0, H3651.B3,0, H3661.B3,0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; no longer C0404.2, C0405.2, C0406.2, C0407.2, C0408.2, C0409.2, C0421.1, C0422.2, C0423.2, C0441.1, C0442.1, C0451.-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
- net MCU_NRST: now also U0101.7; no longer U0111.25
- net MCU_VBAT: now also C0451.1, U0101.1; no longer C0451.+, D1901.A, U0111.6
- net MCU_VDD: now also U0101.19, U0101.32, U0101.64; no longer C0404.1, C0405.1, C0406.1, C0407.1, C0408.1, C0409.1, U0111.108, U0111.121, U0111.144, U0111.17, U0111.39, U0111.52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
- net MCU_VDDA: now also U0101.13; no longer U0111.33
- net MCU_VREF_M: now also U0101.12; no longer U0111.31
- net PA0: now also U0101.14; no longer R2611.2, U0111.34
- net PA1: now also U0101.15; no longer R1543.2, U0111.35
- net PA10: now also U0101.43; no longer U0111.102
- net PA12PA11_N: no longer U0111.103
- net PA12PA11_P: no longer U0111.104
- net PA13: now also U0101.46; no longer U0111.105
- net PA14: now also U0101.49; no longer U0111.109
- net PA15: now also U0101.50; no longer U0111.110
- net PA2: now also U0101.16; no longer R2010.1, U0111.36
- net PA3: now also U0101.17; no longer R2541.1, TP_LIPO_CUR.TP, U0111.37
- net PA4: now also U0101.20; no longer U0111.40
- net PA5: now also U0101.21; no longer R2554.1, U0111.41
- net PA6: now also U0101.22; no longer R2023.2, U0111.42
- net PA7: now also U0101.23; no longer R1122.2, U0111.43
- net PA8: now also U0101.41; no longer U0111.100, U1601.3
- net PA9: now also U0101.42; no longer U0111.101
- net PB0: now also U0101.26; no longer R1132.2, U0111.46
- net PB1: now also U0101.27; no longer R2012.1, U0111.47
- net PB10: now also U0101.29; no longer U0111.69
- net PB12: now also U0101.33; no longer U0111.73
- net PB13: now also U0101.34; no longer R1752.2, R3521.1, R3586.1, U0111.74
- net PB14: now also U0101.35; no longer U0111.75
- net PB15: now also U0101.36; no longer R3514.1, R3579.1, U0111.76
- net PB2: now also U0101.28; no longer U0111.48
- net PB3: now also U0101.55; no longer R3501.1, U0111.132
- net PB4: now also U0101.56; no longer U0111.133
- net PB5: now also U0101.57; no longer R3502.1, U0111.134
- net PB6: now also U0101.58; no longer R3503.1, U0111.135
- net PB7: now also U0101.59; no longer R3504.1, U0111.136
- net PB8: now also U0101.61; no longer U0111.138
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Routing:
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- removed copper zone on layer 2, net BME680_LAYER02_CUTOUT
- removed copper zone on layer 15, net BME680_LAYER15_CUTOUT
- removed copper zone on layer 15, net POLY_BT_1
- removed copper zone on layer 2, net POLY_BT_2
- removed copper zone on layer 15, net POLY_GPS_0
- removed copper zone on layer 15, net POLY_GPS_1
- removed copper zone on layer 2, net POLY_GPS_2
- removed copper zone on layer 1, net POLY_GPS_3
- removed copper zone on layer 1, net POLY_GPS_4
- removed copper zone on layer 15, net POLY_GSM_1
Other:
- board size 96.5 x 96.5 mm -> 96.5 x 73 mm
- board text added: "CAT Ifc."
- board text added: "CTS"
- board text added: "DL0WH BiTuner V1.0 (C) 2019"
- board text added: "FWD"
- board text added: "GND"
- board text added: "REL1..20"
- board text added: "REL21..36, 12V"
- board text added: "REV"
- board text added: "RS232"
- board text added: "RTR"
- board text added: "RXD"
- board text added: "TXD"
- board text added: "USB"
- board text removed: "ADC1"
- board text removed: "ADC2"
- board text removed: "BAT"
- board text removed: "BT"
- board text removed: "C1"
- board text removed: "C2"
- board text removed: "CUR"
- board text removed: "D1"
- board text removed: "D2"
- board text removed: "D3"
- board text removed: "GPIO"
- board text removed: "GPS"
- board text removed: "GSM"
- board text removed: "HFT-Core-Module V1.1 (C) 2018 by Fakultät N, Hochschule Mannheim, Germany."
- board text removed: "HICUR"
- board text removed: "IN"
- board text removed: "IRQ"
- board text removed: "LiPo"
- board text removed: "OUT"
- board text removed: "PMIC_1V2"
- board text removed: "SIM USB"
- board text removed: "SIM-Card"
- board text removed: "SMPS"
- board text removed: "SOLAR"
- board text removed: "SYS"
- board text removed: "USW"
- board text removed: "VBAT"
- board text removed: "VBKUP"
- board text removed: "VOUT"
- board text removed: "VSOL"
- board text removed: "VSTOR"
- board text removed: "XO"
- board text removed: "XO_PA"
